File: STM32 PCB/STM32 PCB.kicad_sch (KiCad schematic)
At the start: 2 parts, among them U1 NUCLEO-L476RG

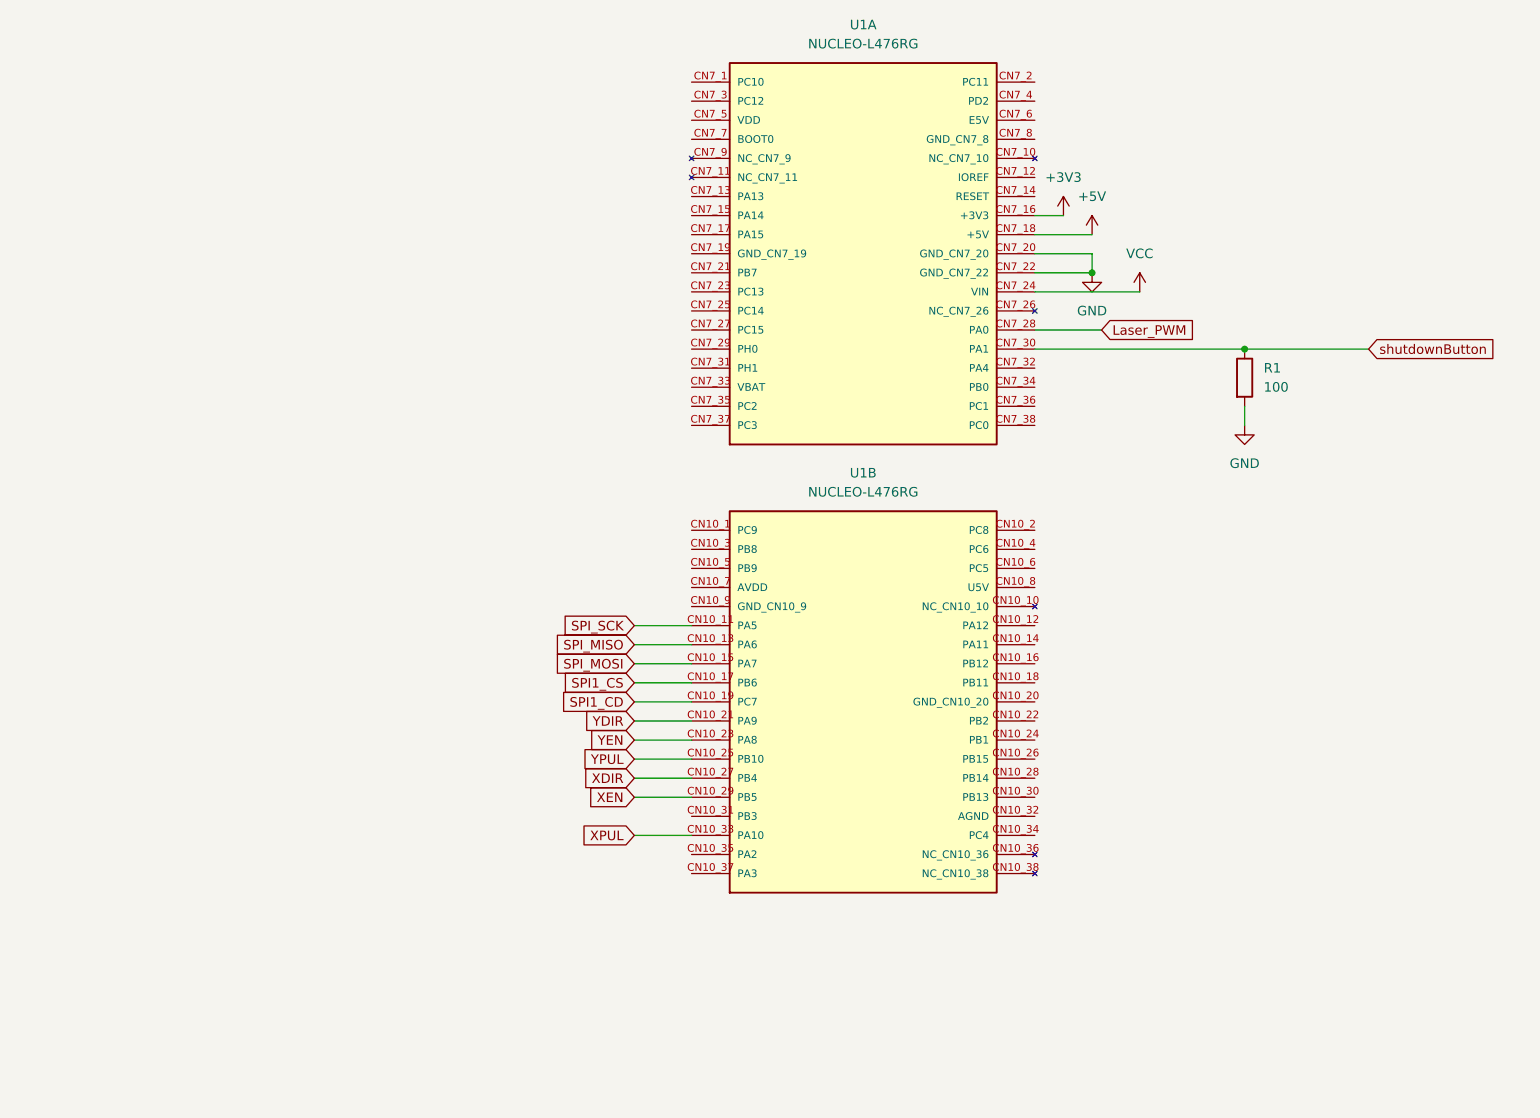
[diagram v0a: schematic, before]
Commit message: PCB upload
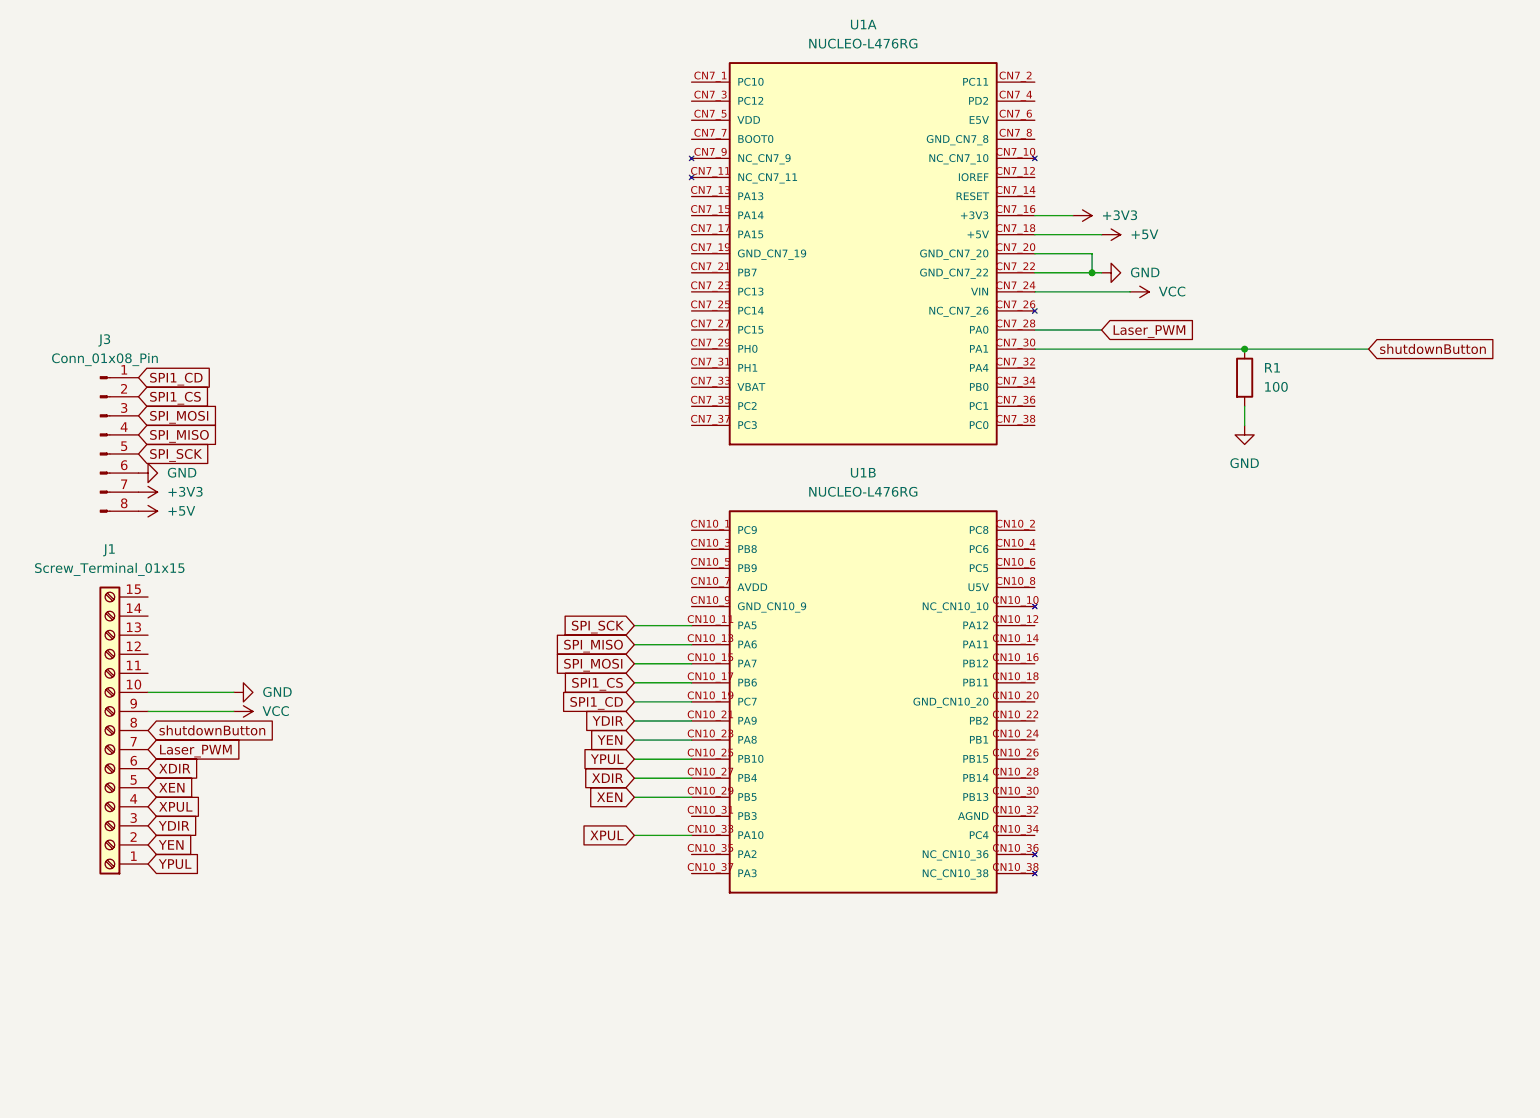
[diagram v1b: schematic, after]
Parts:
- added J1: Screw_Terminal_01x15, Connector_PinSocket_2.54mm:PinSocket_1x15_P2.54mm_Vertical, symbol Connector:Screw_Terminal_01x15
- added J3: Conn_01x08_Pin, Connector_PinSocket_2.54mm:PinSocket_1x08_P2.54mm_Vertical, symbol Connector:Conn_01x08_Pin
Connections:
- net +3V3: now also J3.7 (Pin_7)
- net +5V: now also J3.8 (Pin_8)
- net GND: now also J1.10 (Pin_10), J3.6 (Pin_6)
- net Laser_PWM: now also J1.7 (Pin_7)
- net SPI1_CD: now also J3.1 (Pin_1)
- net SPI1_CS: now also J3.2 (Pin_2)
- net SPI_MISO: now also J3.4 (Pin_4)
- net SPI_MOSI: now also J3.3 (Pin_3)
- net SPI_SCK: now also J3.5 (Pin_5)
- net VCC: now also J1.9 (Pin_9)
- net XDIR: now also J1.6 (Pin_6)
- net XEN: now also J1.5 (Pin_5)
- net XPUL: now also J1.4 (Pin_4)
- net YDIR: now also J1.3 (Pin_3)
- net YEN: now also J1.2 (Pin_2)
- net YPUL: now also J1.1 (Pin_1)
- net shutdownButton: now also J1.8 (Pin_8)

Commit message: PCB updates
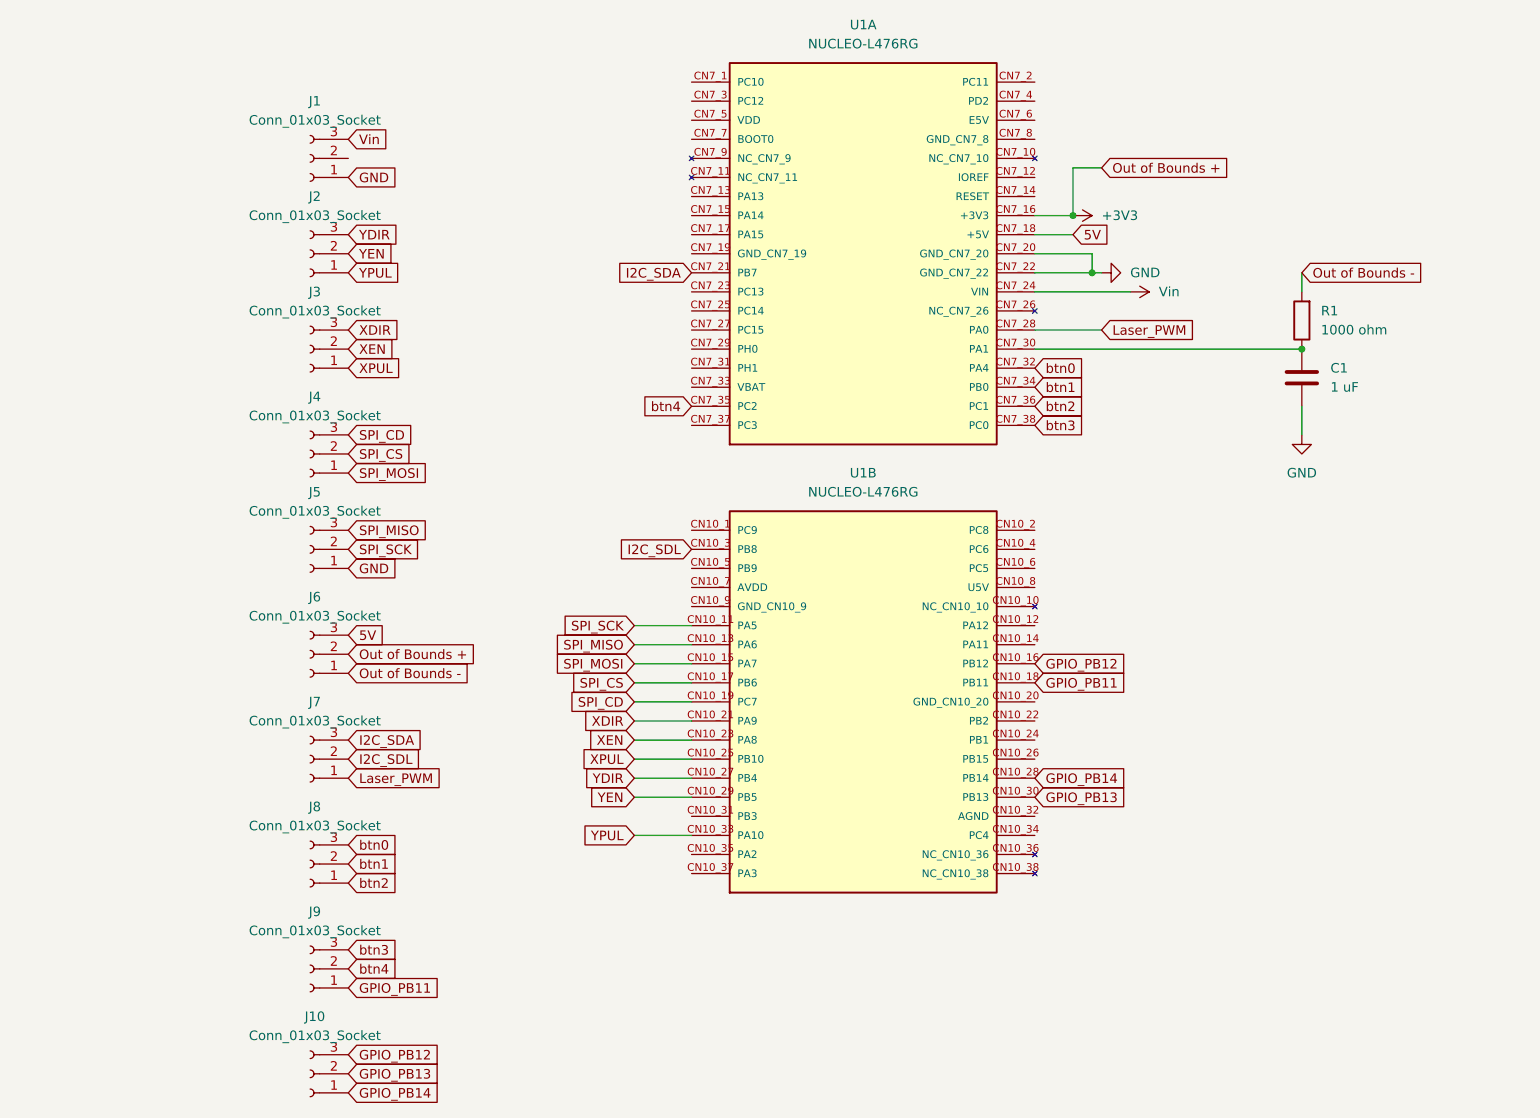
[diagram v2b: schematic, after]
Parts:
- removed J1: Screw_Terminal_01x15, Connector_PinSocket_2.54mm:PinSocket_1x15_P2.54mm_Vertical, symbol Connector:Screw_Terminal_01x15
- removed J3: Conn_01x08_Pin, Connector_PinSocket_2.54mm:PinSocket_1x08_P2.54mm_Vertical, symbol Connector:Conn_01x08_Pin
- added C1: 1 uF, Capacitor_SMD:C_0805_2012Metric_Pad1.18x1.45mm_HandSolder, symbol Device:C
- added J1, J10, J2, J3, J4, J5, J6, J7, J8, J9: Conn_01x03_Socket, Connector_PinHeader_2.54mm:PinHeader_1x03_P2.54mm_Vertical, symbol Connector:Conn_01x03_Socket
- R1: value 100 -> 1000 ohm; footprint Resistor_THT:R_Axial_DIN0411_L9.9mm_D3.6mm_P12.70mm_Horizontal -> Resistor_SMD:R_0805_2012Metric_Pad1.20x1.40mm_HandSolder
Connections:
- net +3V3: now also J6.2 (Pin_2)
- net GND: now also C1.1, J1.1 (Pin_1), J5.1 (Pin_1); no longer R1.2
- net Laser_PWM: now also J7.1 (Pin_1)
- net SPI_MISO: now also J5.3 (Pin_3)
- net SPI_MOSI: now also J4.1 (Pin_1)
- net SPI_SCK: now also J5.2 (Pin_2)
- net XDIR: now also U1.CN10_21 (PA9), J3.3 (Pin_3); no longer U1.CN10_27 (PB4)
- net XEN: now also U1.CN10_23 (PA8), J3.2 (Pin_2); no longer U1.CN10_29 (PB5)
- net XPUL: now also U1.CN10_25 (PB10), J3.1 (Pin_1); no longer U1.CN10_33 (PA10)
- net YDIR: now also U1.CN10_27 (PB4), J2.3 (Pin_3); no longer U1.CN10_21 (PA9)
- net YEN: now also U1.CN10_29 (PB5), J2.2 (Pin_2); no longer U1.CN10_23 (PA8)
- net YPUL: now also U1.CN10_33 (PA10), J2.1 (Pin_1); no longer U1.CN10_25 (PB10)
- net I2C_SDA: now reaches U1.CN7_21 (PB7)
- net I2C_SDA: now also J7.3 (Pin_3)
- net btn0: now reaches U1.CN7_32 (PA4)
- net btn0: now also J8.3 (Pin_3)
- net btn1: now reaches U1.CN7_34 (PB0)
- net btn1: now also J8.2 (Pin_2)
- net btn4: now reaches U1.CN7_35 (PC2)
- net btn4: now also J9.2 (Pin_2)
- net btn2: now reaches U1.CN7_36 (PC1)
- net btn2: now also J8.1 (Pin_1)
- net btn3: now reaches U1.CN7_38 (PC0)
- net btn3: now also J9.3 (Pin_3)
- net GPIO_PB12: now reaches U1.CN10_16 (PB12)
- net GPIO_PB12: now also J10.3 (Pin_3)
- net GPIO_PB11: now reaches U1.CN10_18 (PB11)
- net GPIO_PB11: now also J9.1 (Pin_1)
- net GPIO_PB14: now reaches U1.CN10_28 (PB14)
- net GPIO_PB14: now also J10.1 (Pin_1)
- net I2C_SDL: now reaches U1.CN10_3 (PB8)
- net I2C_SDL: now also J7.2 (Pin_2)
- net GPIO_PB13: now reaches U1.CN10_30 (PB13)
- net GPIO_PB13: now also J10.2 (Pin_2)
- net +5V renamed 5V
- net 5V: now also J6.3 (Pin_3)
- net SPI1_CD renamed SPI_CD
- net SPI_CD: now also J4.3 (Pin_3)
- net SPI1_CS renamed SPI_CS
- net SPI_CS: now also J4.2 (Pin_2)
- net VCC renamed Vin
- net Vin: now also J1.3 (Pin_3)
- net shutdownButton: no longer names the net of R1.1, U1.CN7_30 (PA1)
- net shutdownButton: now also C1.2
- new net Out of Bounds -: J6.1 (Pin_1), R1.2
